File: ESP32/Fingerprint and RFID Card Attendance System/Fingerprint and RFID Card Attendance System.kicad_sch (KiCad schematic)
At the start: 9 parts, among them J1 128X64 2.42 INCH OLED SCREEN, J2 AS608

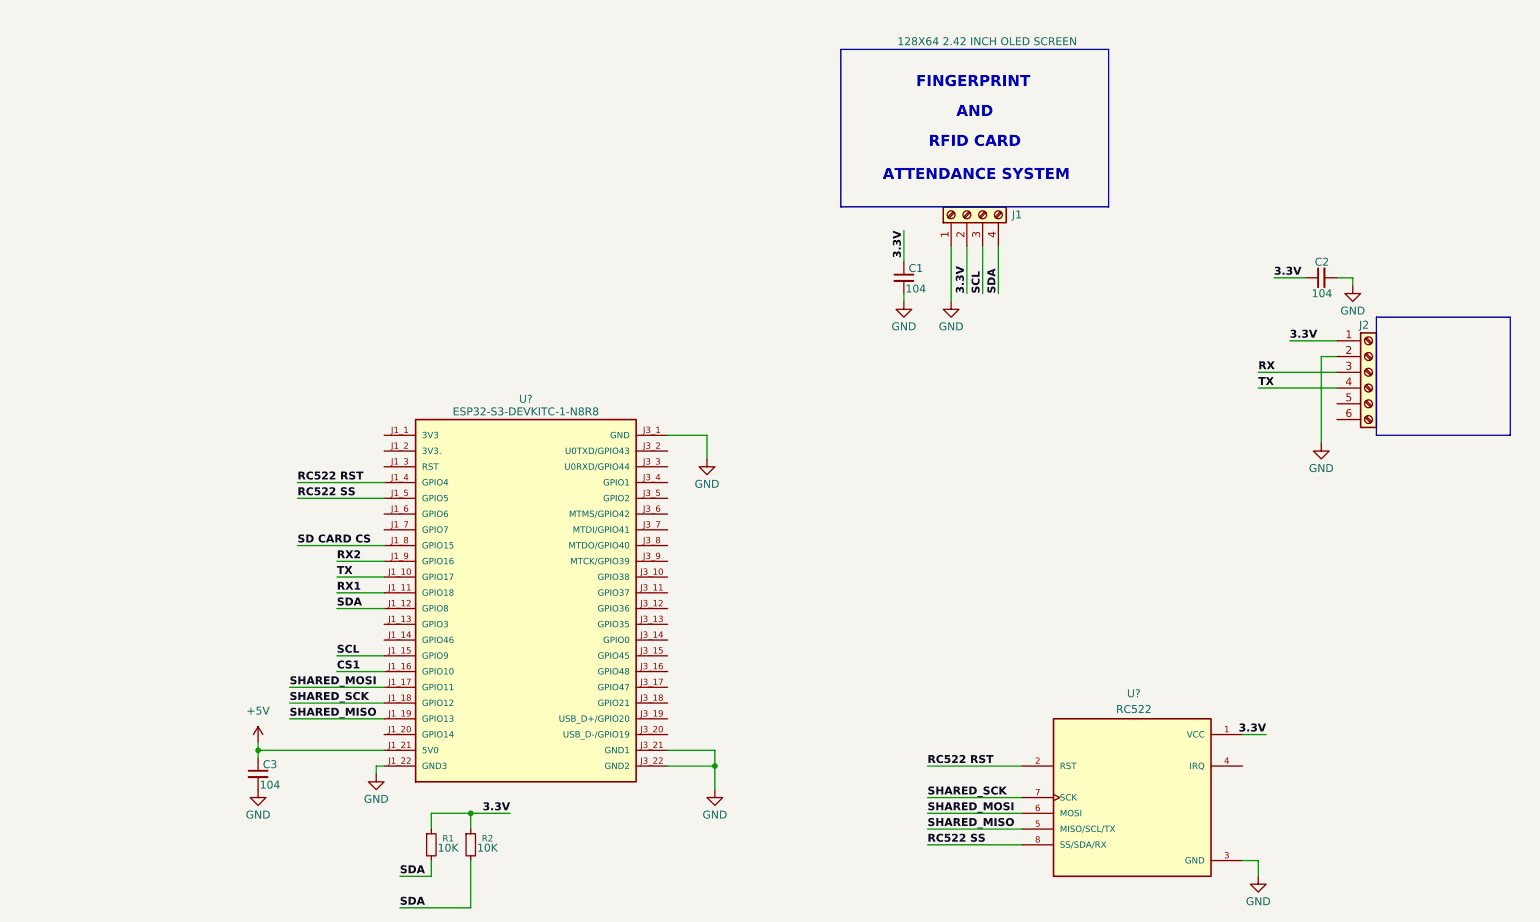
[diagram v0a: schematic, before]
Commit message: done with schematic and block diagram
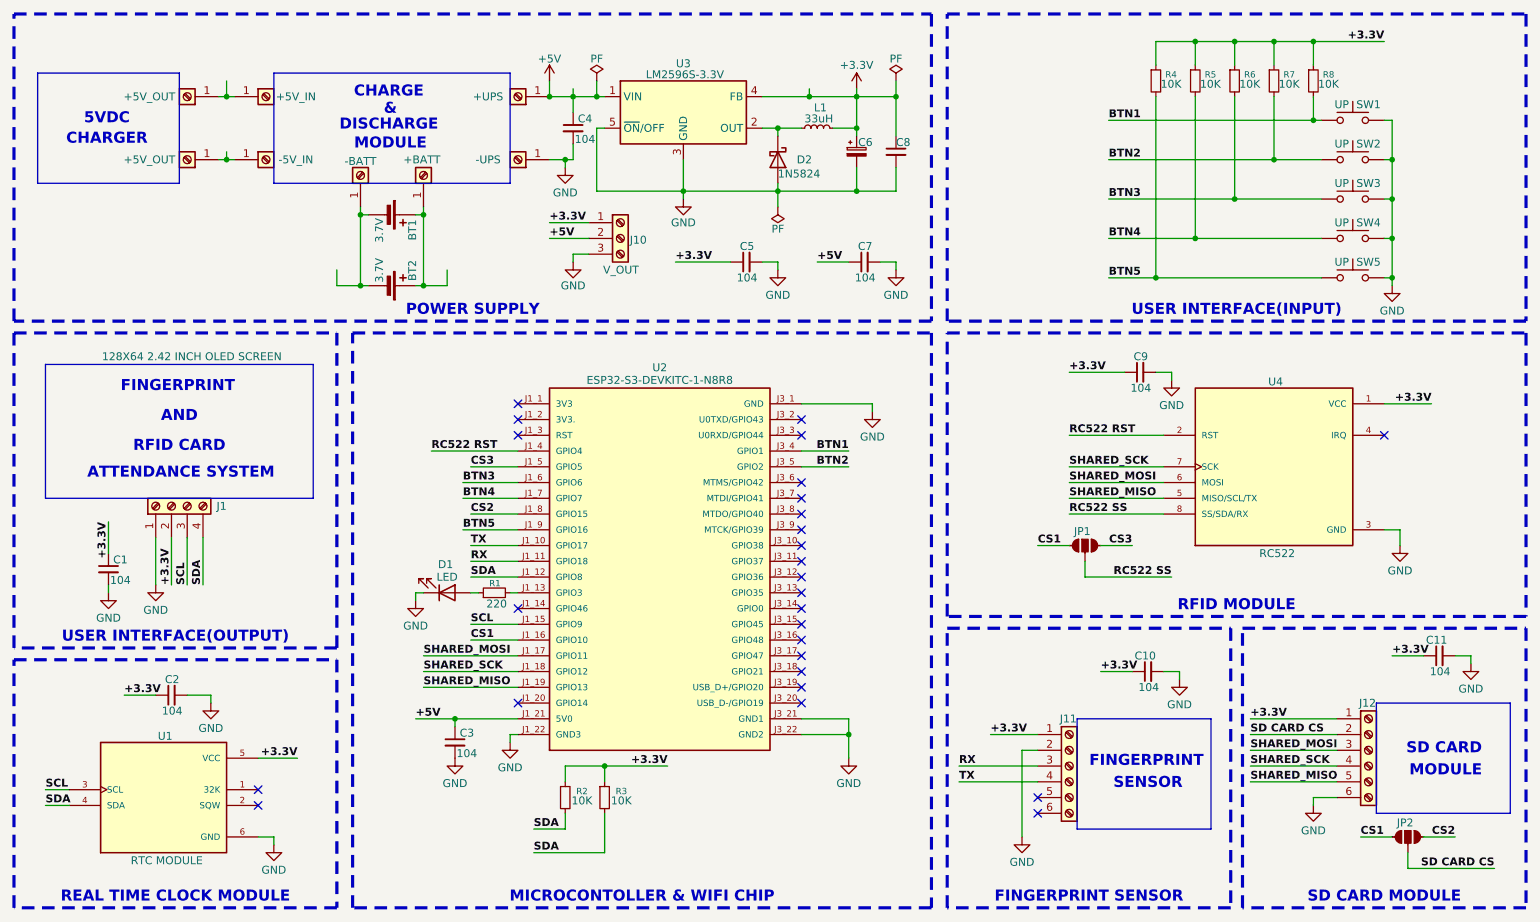
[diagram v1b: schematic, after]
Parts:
- added BT1, BT2: 3.7V, symbol Device:Battery_Cell
- added C11, C2, C4, C5, C7, C9: 104, symbol Device:C_Small
- added C6: 220uF_16V, Capacitor_THT:CP_Radial_D8.0mm_P3.80mm, symbol Device:C_Polarized_Small
- added C8: 100nF, Capacitor_THT:C_Disc_D5.1mm_W3.2mm_P5.00mm, symbol Device:C_Small
- added D1: LED, symbol Device:LED
- added D2: 1N5824, Diode_SMD:D_2010_5025Metric, symbol Diode:1N5822
- added J10: V_OUT, symbol Connector:Screw_Terminal_01x03
- added J12: AS608, symbol Connector:Screw_Terminal_01x06
- added J2, J3: +5V_OUT, symbol Connector:Screw_Terminal_01x01
- added J4: +5V_IN, symbol Connector:Screw_Terminal_01x01
- added J5: -5V_IN, symbol Connector:Screw_Terminal_01x01
- added J6: -BATT, symbol Connector:Screw_Terminal_01x01
- added J7: +BATT, symbol Connector:Screw_Terminal_01x01
- added J8: +UPS, symbol Connector:Screw_Terminal_01x01
- added J9: -UPS, symbol Connector:Screw_Terminal_01x01
- added JP1, JP2: ~, PCM_SparkFun-Jumper:Jumper_3_NO, symbol PCM_SparkFun-Jumper:SolderJumper_3_Open
- added L1: 33uH, Inductor_SMD:L_12x12mm_H4.5mm, symbol Device:L_Small
- added R1: 220, symbol Device:R_Small
- added R4, R5, R6, R7, R8: 10K, symbol Device:R_Small
- added SW1, SW2, SW3, SW4, SW5: UP, symbol Switch:SW_Push
- added U1: RTC MODULE, TC00500:MODULE_TC00500, symbol RTC:TC00500
- added U3: LM2596S-3.3V, Package_TO_SOT_SMD:TO-263-5_TabPin3, symbol Regulator_Switching:LM2596S-5
- gave numbers to parts that had none: 2
- renumbered C2 to C10, J2 to J11, R1 to R2, R2 to R3
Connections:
- net RX1 is gone; now on net RX: U2.J1_11 (GPIO18)
- net +5V: now also C4.1, C7.1, J10.2 (Pin_2), J8.1 (Pin_1), U3.1 (VIN)
- net CS1: now also JP1.1 (A), JP2.1 (A)
- net GND: now also C11.2, C2.2, C4.2, C5.2, C6.2, C7.2, C8.2, C9.2, D1.1 (K), D2.2 (A), J10.3 (Pin_3), J12.6 (Pin_6), J9.1 (Pin_1), SW1.2, SW2.2, SW3.2, SW4.2, SW5.2, U1.6 (GND), U3.3 (GND), U3.5 (~{ON}/OFF)
- net RC522 SS: now also JP1.2 (B); no longer U2.J1_5 (GPIO5)
- net SCL: now also U1.3 (SCL)
- net SD CARD CS: now also J12.2 (Pin_2), JP2.2 (B); no longer U2.J1_8 (GPIO15)
- net SDA: now also U1.4 (SDA)
- net SHARED_MISO: now also J12.5 (Pin_5)
- net SHARED_MOSI: now also J12.3 (Pin_3)
- net SHARED_SCK: now also J12.4 (Pin_4)
- net at U2.J1_13 (GPIO3): now also R1.2
- net BTN3: now reaches U2.J1_6 (GPIO6)
- net BTN3: now also R6.2, SW3.1
- net BTN4: now reaches U2.J1_7 (GPIO7)
- net BTN4: now also R5.2, SW4.1
- net BTN1: now reaches U2.J3_4 (GPIO1)
- net BTN1: now also R8.2, SW1.1
- net BTN2: now reaches U2.J3_5 (GPIO2)
- net BTN2: now also R7.2, SW2.1
- net 3.3V renamed +3.3V
- net +3.3V: now also C11.1, C2.1, C5.1, C6.1, C8.1, C9.1, J10.1 (Pin_1), J12.1 (Pin_1), L1.2, R4.1, R5.1, R6.1, R7.1, R8.1, U1.5 (VCC), U3.4 (FB)
- net RX2 renamed BTN5
- net BTN5: now also R4.2, SW5.1
- new net: D2.1 (K), L1.1, U3.2 (OUT)
- new net: D1.2 (A), R1.1
- new net: J2.1 (Pin_1), J4.1 (Pin_1)
- new net: J3.1 (Pin_1), J5.1 (Pin_1)
- new net: BT1.1 (+), BT2.1 (+), J7.1 (Pin_1)
- new net: BT1.2 (-), BT2.2 (-), J6.1 (Pin_1)
- new net CS2: JP2.3 (C), U2.J1_8 (GPIO15)
- new net CS3: JP1.3 (C), U2.J1_5 (GPIO5)
- no-connect marks 0 -> 27
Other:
- note added: "&"
- note added: "5VDC"
- note added: "CHARGE"
- note added: "CHARGER"
- note added: "DISCHARGE"
- note added: "MODULE"
- note added: "SD CARD"
- note added: "SENSOR"
- moved on the sheet: C1, C10, C3, J1, J11, R2, R3, U2, U4
